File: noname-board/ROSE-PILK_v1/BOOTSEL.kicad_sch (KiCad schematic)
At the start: 2 parts, among them SW2 SW_Push_Dual

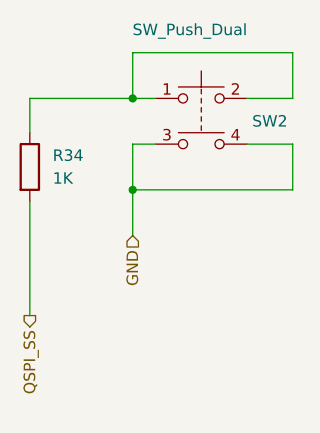
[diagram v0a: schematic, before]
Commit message: Meeting Stuff
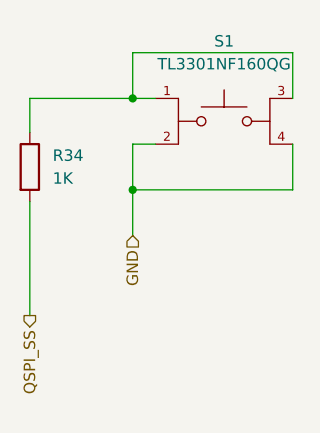
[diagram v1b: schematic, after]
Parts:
- removed SW2: SW_Push_Dual, Button_Switch_THT:SW_CuK_JS202011CQN_DPDT_Straight, symbol Switch:SW_Push_Dual
- added S1: TL3301NF160QG, TL3301NF160QG:SW_TL3301NF160QG, symbol TL3301NF160QG:TL3301NF160QG
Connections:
- net GND: now also S1.2, S1.4
- net at R34.1: now also S1.1, S1.3
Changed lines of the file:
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@@
-    (stroke (width 0) (type default))
-  )
-  (wire (pts (xy 147.32 50.8) (xy 152.4 50.8))
     (stroke (width 0) (type default))
   )
   (wire (pts (xy 134.62 45.72) (xy 134.62 50.8))
-    (stroke (width 0) (type default))
-  )
-  (wire (pts (xy 147.32 55.88) (xy 152.4 55.88))
     (stroke (width 0) (type default))
   )
@@
     )
   )
-  (symbol (lib_id "Switch:SW_Push_Dual") (at 142.24 50.8 0) (unit 1)
-    (in_bom yes) (on_board yes) (dnp no)
-    (property "Reference" "SW2" (at 149.86 53.34 0)
+  (symbol (lib_id "TL3301NF160QG:TL3301NF160QG") (at 144.78 53.34 0) (unit 1)
+    (in_bom yes) (on_board yes) (dnp no) (fields_autoplaced)
+    (property "Reference" "S1" (at 144.78 44.45 0)
       (effects (font (size 1.27 1.27)))
     )
-    (property "Value" "SW_Push_Dual" (at 140.97 43.18 0)
+    (property "Value" "TL3301NF160QG" (at 144.78 46.99 0)
       (effects (font (size 1.27 1.27)))
     )
-    (property "Footprint" "Button_Switch_THT:SW_CuK_JS202011CQN_DPDT_Straight" (at 142.24 45.72 0)
+    (property "Footprint" "TL3301NF160QG:SW_TL3301NF160QG" (at 144.78 53.34 0)
+      (effects (font (size 1.27 1.27)) (justify bottom) hide)
+    )
+    (property "Datasheet" "" (at 144.78 53.34 0)
       (effects (font (size 1.27 1.27)) hide)
     )
-    (property "Datasheet" "~" (at 142.24 45.72 0)
-      (effects (font (size 1.27 1.27)) hide)
+    (property "MF" "E-Switch" (at 144.78 53.34 0)
+      (effects (font (size 1.27 1.27)) (justify bottom) hide)
+    )
+    (property "Purchase-URL" "https://www.snapeda.com/api/url_track_click_mouser/?unipart_id=304402&manufacturer=E-Switch&part_name=TL3301NF160QG&search_term=None" (at 144.78 53.34 0)
+      (effects (font (size 1.27 1.27)) (justify bottom) hide)
+    )
+    (property "Package" "None" (at 144.78 53.34 0)
+      (effects (font (size 1.27 1.27)) (justify bottom) hide)
+    )
+    (property "Price" "None" (at 144.78 53.34 0)
+      (effects (font (size 1.27 1.27)) (justify bottom) hide)
+    )
+    (property "Check_prices" "https://www.snapeda.com/parts/TL3301NF160QG/E-Switch/view-part/?ref=eda" (at 144.78 53.34 0)
+      (effects (font (size 1.27 1.27)) (justify bottom) hide)
+    )
+    (property "SnapEDA_Link" "https://www.snapeda.com/parts/TL3301NF160QG/E-Switch/view-part/?ref=snap" (at 144.78 53.34 0)
+      (effects (font (size 1.27 1.27)) (justify bottom) hide)
+    )
+    (property "MP" "TL3301NF160QG" (at 144.78 53.34 0)
+      (effects (font (size 1.27 1.27)) (justify bottom) hide)
+    )
+    (property "Availability" "In Stock" (at 144.78 53.34 0)
+      (effects (font (size 1.27 1.27)) (justify bottom) hide)
+    )
+    (property "Description" "\nTactile Switch, TL3301, SPST-NO, OFF-(ON), 4.3mm Top Actuated, 0.05A, 12VDC | E-Switch TL3301NF160QG\n" (at 144.78 53.34 0)
+      (effects (font (size 1.27 1.27)) (justify bottom) hide)
     )
     (pin "1")
@@
     (instances
       (project "ROSE-PILK_v1"
-        (path "/3dfb9737-68ba-4ca9-8085-72e4f57f9e50/0210b5e9-62f8-4096-ad3b-68b9f2dd9ed6"
-          (reference "SW2") (unit 1)
-        )
         (path "/3dfb9737-68ba-4ca9-8085-72e4f57f9e50/ee4b99aa-294b-4c3b-9b79-fbaf11f9a74b"
-          (reference "SW3") (unit 1)
+          (reference "S1") (unit 1)
         )
       )
